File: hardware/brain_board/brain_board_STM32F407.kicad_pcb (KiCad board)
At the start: 2 copper layers, 61.8 x 73.2 mm, 70 parts, among them J1 MINI-USB-5P-3400020P1, J2 MINI-USB-5P-3400020P1V, P1 CONN_25X2, P2 CONN_25X2, P3 CONN_2, P4 CONN_02X05, P5 CONN_01X03, P6 CONN_01X03, SW1 SW_PUSH, SW2 SW_PUSH, U1 STM32F407VG, U2 NUF2101MT1G, U3 LM2937, X1 CRYSTAL, X2 CRYSTAL(MC306)

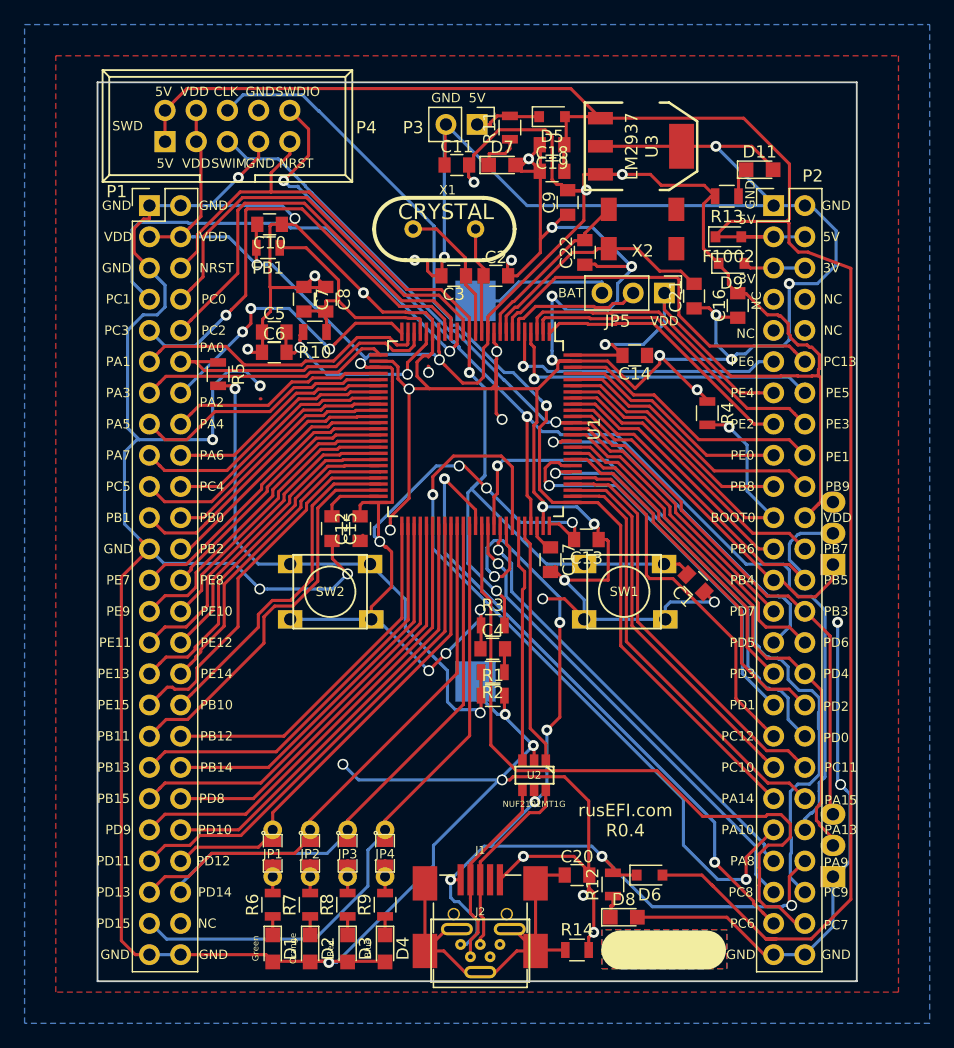
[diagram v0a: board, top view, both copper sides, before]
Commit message: update pcb files
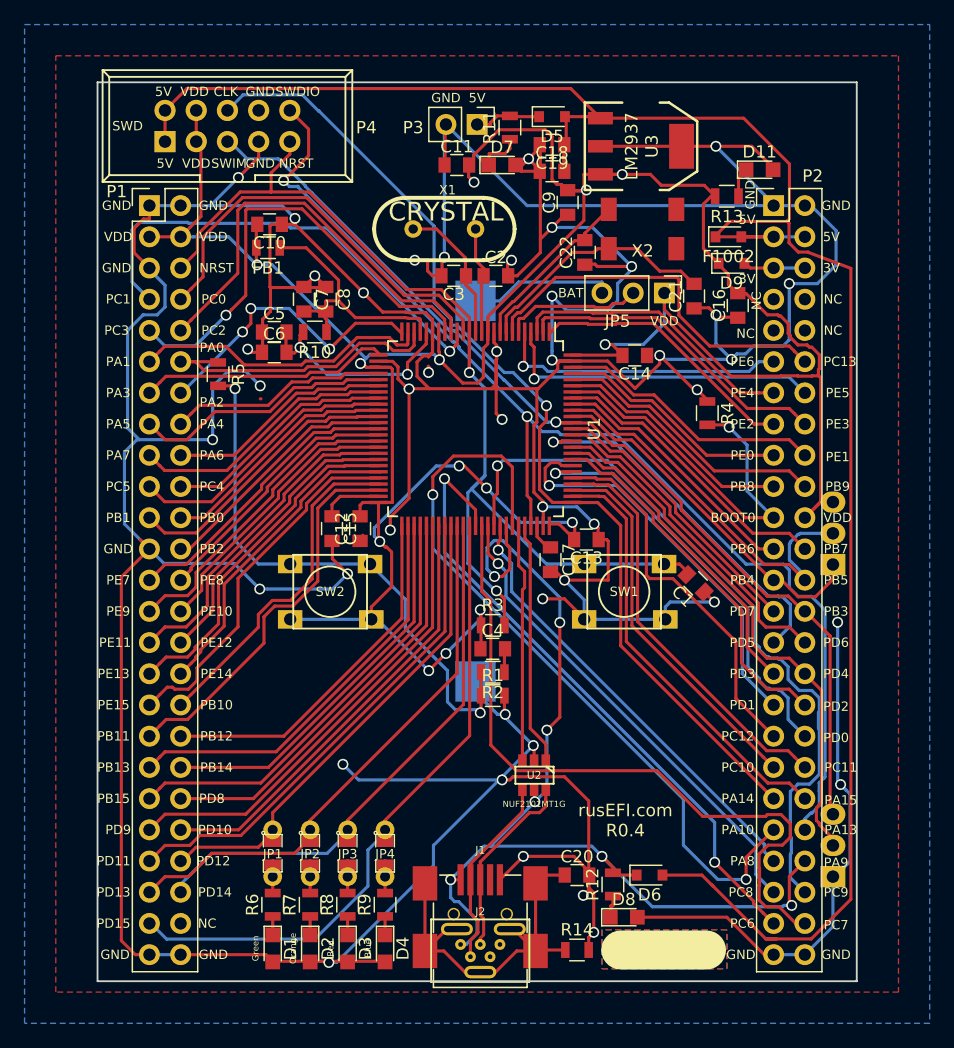
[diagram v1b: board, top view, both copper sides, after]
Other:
- net class Default removed
